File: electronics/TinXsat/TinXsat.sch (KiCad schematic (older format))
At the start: 159 parts, among them J1 USB_B_Mini, J10 CAN, J2 ESP-PROG, J3 POWER_LED, J4 MCO_OUT, J5 BMP280_1, J6 BMP280_2, J7 ESP-card, J8 GPS, J9 SWD, Q1 Si2371, Q2 Si2371, Q3 BSS138, Q4 BSS138, Q5 Si2371, Q6 BSS138, Q7 BSS138, Q8 STD7NK40Z, SW1 SW_Push, U1 CP2102N-A01-GQFN28, U10 TPS61175PWP, U11 STM32F103RGTx, U12 LM35-LP, U13 LM35-LP, U14 LM35-LP, U15 TPS63001, U2 A25L032, U3 MPU-6050, U4 TP4056, U5 Ai-Thinker-Ra-01, U6 ESP32-cam, U7 INA219AxDCN, U8 MCP130, U9 INA219AxDCN, Y1 8Mhz, Y2 32768Hz

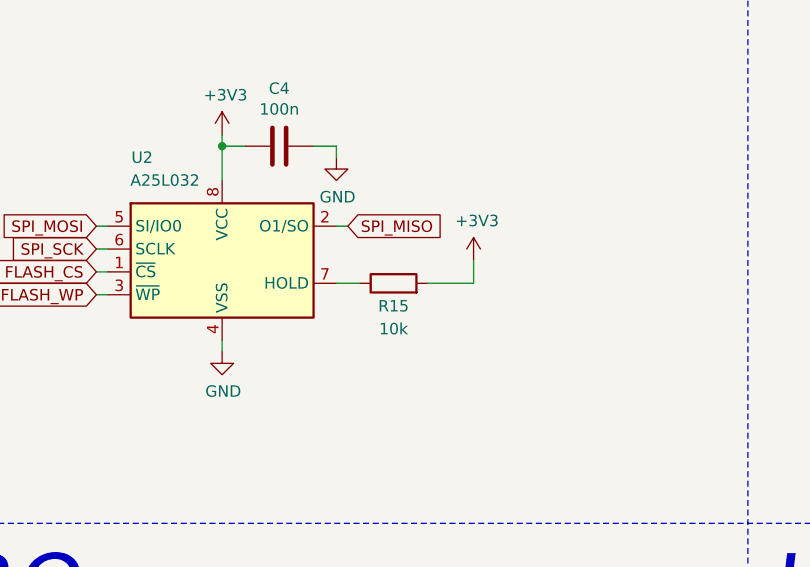
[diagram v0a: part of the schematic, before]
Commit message: pcb gerber commit
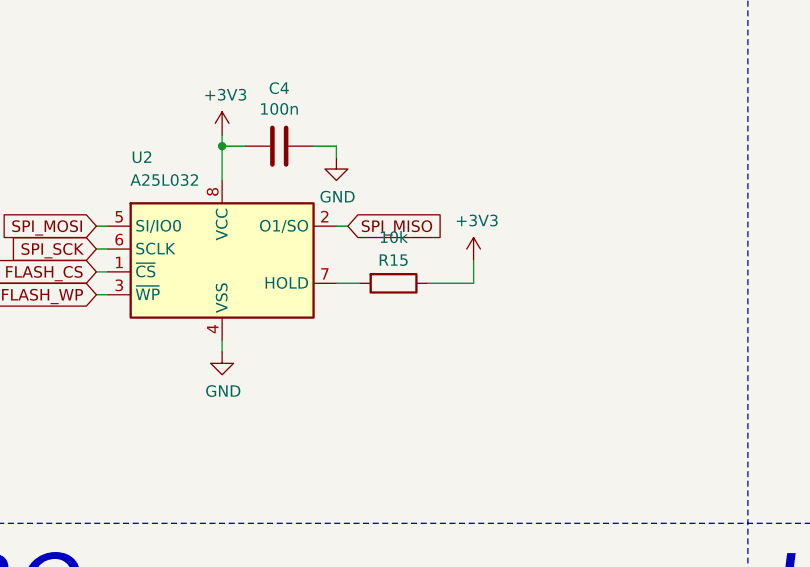
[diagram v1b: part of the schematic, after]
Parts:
- U2: footprint Package_SO:SOP-8_3.9x4.9mm_P1.27mm -> TinXsat:WSON-8-1EP_6x5mm_P1.27mm_EP3.4x4mm
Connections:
- net +3V3: now also R15.1; no longer R15.2
- net at U2.7 (HOLD): now also R15.2; no longer R15.1
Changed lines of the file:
@@
 FLASH_WP
-$Comp
-L sch-lib:A25L032 U2
-U 1 1 60070B82
-P 2250 6750
-F 0 "U2" H 1900 7250 50  0000 C CNN
-F 1 "A25L032" H 2000 7150 50  0000 C CNN
-F 2 "Package_SO:SOP-8_3.9x4.9mm_P1.27mm" H 2250 6150 50  0001 C CNN
-F 3 "http://www.elm-tech.com/en/products/spi-flash-memory/gd25d10/gd25d10.pdf" H 2250 6750 50  0001 C CNN
-	1    2250 6750
-	1    0    0    -1
-$EndComp
 $Comp
 L power:GND #PWR0162
@@
 	1700 6750 1750 6750
 $Comp
-L Device:R R15
-U 1 1 60255FDC
-P 3000 6800
-F 0 "R15" V 2900 6800 50  0000 C CNN
-F 1 "10k" V 2800 6800 50  0000 C CNN
-F 2 "Resistor_SMD:R_0805_2012Metric_Pad1.20x1.40mm_HandSolder" V 2930 6800 50  0001 C CNN
-F 3 "~" H 3000 6800 50  0001 C CNN
-	1    3000 6800
-	0    -1   -1   0
-$EndComp
-$Comp
 L power:+3V3 #PWR0159
 U 1 1 60256D6F
@@
 Wire Wire Line
 	3350 6700 3350 6800
-Wire Wire Line
-	3350 6800 3150 6800
-Wire Wire Line
-	2850 6800 2750 6800
 Wire Wire Line
 	1700 6850 1750 6850
@@
 Wire Wire Line
 	21300 13600 21300 13800
+$Comp
+L Device:R R15
+U 1 1 60130731
+P 3000 6800
+F 0 "R15" V 2900 6800 50  0000 C CNN
+F 1 "10k" V 2800 6800 50  0000 C CNN
+F 2 "Resistor_SMD:R_0805_2012Metric_Pad1.20x1.40mm_HandSolder" V 2930 6800 50  0001 C CNN
+F 3 "~" H 3000 6800 50  0001 C CNN
+	1    3000 6800
+	0    1    1    0
+$EndComp
+Wire Wire Line
+	3150 6800 3350 6800
+Wire Wire Line
+	2750 6800 2850 6800
+$Comp
+L sch-lib:A25L032 U2
+U 1 1 60070B82
+P 2250 6750
+F 0 "U2" H 1900 7250 50  0000 C CNN
+F 1 "A25L032" H 2000 7150 50  0000 C CNN
+F 2 "TinXsat:WSON-8-1EP_6x5mm_P1.27mm_EP3.4x4mm" H 2250 6150 50  0001 C CNN
+F 3 "http://www.elm-tech.com/en/products/spi-flash-memory/gd25d10/gd25d10.pdf" H 2250 6750 50  0001 C CNN
+	1    2250 6750
+	1    0    0    -1
+$EndComp
 $EndSCHEMATC

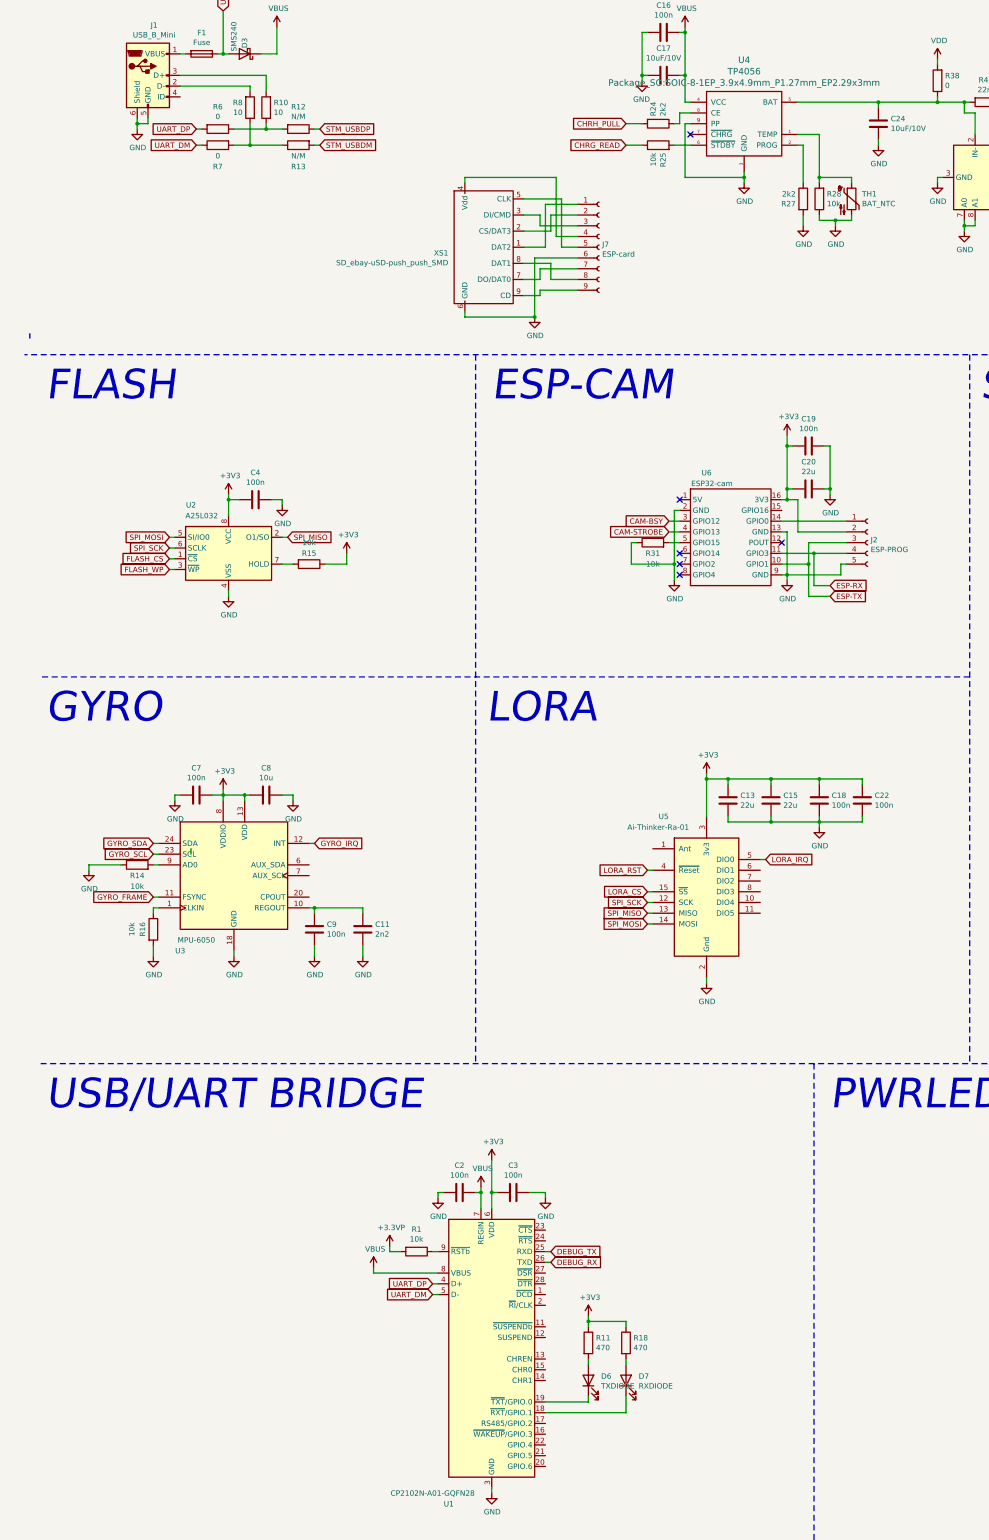
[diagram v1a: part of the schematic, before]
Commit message: pcb final commit after chinese changes
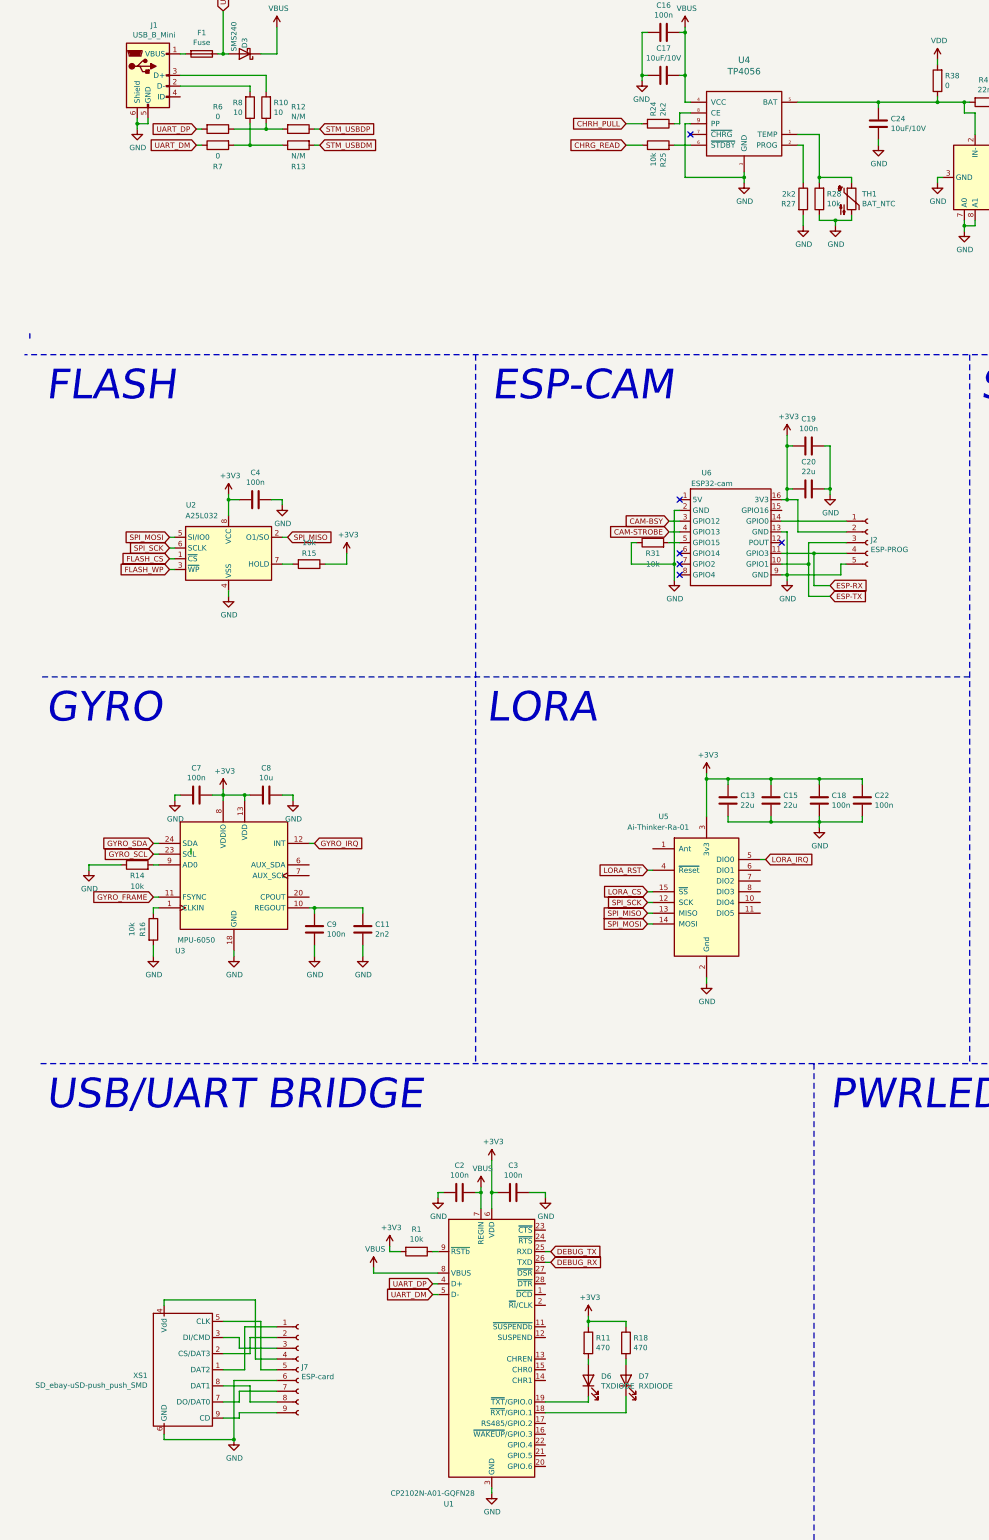
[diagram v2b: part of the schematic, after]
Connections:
- net +3.3VP is gone; now on net +3V3: R1.2
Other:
- moved on the sheet: J7, XS1
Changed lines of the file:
@@
 	4700 12350 4700 12650
 Connection ~ 4700 12650
-$Comp
-L power:+3.3VP #PWR0201
-U 1 1 61CD4E41
-P 3750 13150
-F 0 "#PWR0201" H 3900 13100 50  0001 C CNN
-F 1 "+3.3VP" H 3765 13323 50  0000 C CNN
-F 2 "" H 3750 13150 50  0001 C CNN
-F 3 "" H 3750 13150 50  0001 C CNN
-	1    3750 13150
-	1    0    0    -1
-$EndComp
 Wire Wire Line
 	4150 13200 4200 13200
@@
 F 0 "U4" H 7050 3393 60  0000 C CNN
 F 1 "TP4056" H 7050 3287 60  0000 C CNN
-F 2 "Package_SO:SOIC-8-1EP_3.9x4.9mm_P1.27mm_EP2.29x3mm" H 7050 3181 60  0000 C CNN
+F 2 "Package_SO:SOIC-8-1EP_3.9x4.9mm_P1.27mm_EP2.29x3mm" H 7050 3181 60  0001 C CNN
 F 3 "" H 7050 2750 60  0000 C CNN
 	1    7050 2750
@@
 	20900 11900 21550 11900
 $Comp
-L uSD_push-push_ebay:SD_ebay-uSD-push_push_SMD XS1
-U 1 1 61BF60BB
-P 4600 3950
-F 0 "XS1" H 4296 3996 50  0000 R CNN
-F 1 "SD_ebay-uSD-push_push_SMD" H 4296 3905 50  0000 R CNN
-F 2 "footprints:Conn_uSDcard" H 4600 3950 10  0001 C CNN
-F 3 "_" H 4600 3950 10  0001 C CNN
-F 4 "_" H 4600 3950 10  0001 C CNN "Manf#"
-F 5 "ebay" H 4600 3950 10  0001 C CNN "Manf"
-	1    4600 3950
-	1    0    0    -1
-$EndComp
-$Comp
 L Analog_ADC:INA219AxDCN U7
 U 1 1 6237EB1E
@@
 L Connector:Conn_01x09_Female J7
 U 1 1 5FEDD748
-P 5700 3850
-F 0 "J7" H 5728 3876 50  0000 L CNN
-F 1 "ESP-card" H 5728 3785 50  0000 L CNN
-F 2 "TinXsat:PinHeader_1x08_P2mm_SMD" H 5700 3850 50  0001 C CNN
-F 3 "~" H 5700 3850 50  0001 C CNN
-	1    5700 3850
-	1    0    0    -1
-$EndComp
-Wire Wire Line
-	5200 3450 5200 3850
-Wire Wire Line
-	5200 3850 5000 3850
-Wire Wire Line
-	5200 3450 5500 3450
-Wire Wire Line
-	5500 3550 5250 3550
-Wire Wire Line
-	5250 3550 5250 3700
-Wire Wire Line
-	5250 3700 5000 3700
-Wire Wire Line
-	5000 3550 5150 3550
-Wire Wire Line
-	5150 3550 5150 3650
-Wire Wire Line
-	5150 3650 5500 3650
-Wire Wire Line
-	4450 3250 4450 3200
-Wire Wire Line
-	4450 3200 5300 3200
-Wire Wire Line
-	5300 3200 5300 3750
-Wire Wire Line
-	5300 3750 5500 3750
-Wire Wire Line
-	5500 3850 5350 3850
-Wire Wire Line
-	5350 3850 5350 3400
-Wire Wire Line
-	5350 3400 5000 3400
-Wire Wire Line
-	4450 4450 4450 4500
-Wire Wire Line
-	4450 4500 5100 4500
-Wire Wire Line
-	5100 4500 5100 3950
-Wire Wire Line
-	5100 3950 5500 3950
-Wire Wire Line
-	5500 4050 5150 4050
-Wire Wire Line
-	5150 4050 5150 4150
-Wire Wire Line
-	5150 4150 5000 4150
-Wire Wire Line
-	5000 4000 5250 4000
-Wire Wire Line
-	5250 4000 5250 4150
-Wire Wire Line
-	5250 4150 5500 4150
-Wire Wire Line
-	5500 4250 5150 4250
-Wire Wire Line
-	5150 4250 5150 4300
-Wire Wire Line
-	5150 4300 5000 4300
+P 2900 14300
+F 0 "J7" H 2928 14326 50  0000 L CNN
+F 1 "ESP-card" H 2928 14235 50  0000 L CNN
+F 2 "TinXsat:PinHeader_1x08_P2mm_SMD" H 2900 14300 50  0001 C CNN
+F 3 "~" H 2900 14300 50  0001 C CNN
+	1    2900 14300
+	1    0    0    -1
+$EndComp
+Wire Wire Line
+	2400 13900 2400 14300
+Wire Wire Line
+	2400 14300 2200 14300
+Wire Wire Line
+	2400 13900 2700 13900
+Wire Wire Line
+	2700 14000 2450 14000
+Wire Wire Line
+	2450 14000 2450 14150
+Wire Wire Line
+	2450 14150 2200 14150
+Wire Wire Line
+	2200 14000 2350 14000
+Wire Wire Line
+	2350 14000 2350 14100
+Wire Wire Line
+	2350 14100 2700 14100
+Wire Wire Line
+	1650 13700 1650 13650
+Wire Wire Line
+	1650 13650 2500 13650
+Wire Wire Line
+	2500 13650 2500 14200
+Wire Wire Line
+	2500 14200 2700 14200
+Wire Wire Line
+	2700 14300 2550 14300
+Wire Wire Line
+	2550 14300 2550 13850
+Wire Wire Line
+	2550 13850 2200 13850
+Wire Wire Line
+	1650 14900 1650 14950
+Wire Wire Line
+	1650 14950 2300 14950
+Wire Wire Line
+	2300 14950 2300 14400
+Wire Wire Line
+	2300 14400 2700 14400
+Wire Wire Line
+	2700 14500 2350 14500
+Wire Wire Line
+	2350 14500 2350 14600
+Wire Wire Line
+	2350 14600 2200 14600
+Wire Wire Line
+	2200 14450 2450 14450
+Wire Wire Line
+	2450 14450 2450 14600
+Wire Wire Line
+	2450 14600 2700 14600
+Wire Wire Line
+	2700 14700 2350 14700
+Wire Wire Line
+	2350 14700 2350 14750
+Wire Wire Line
+	2350 14750 2200 14750
 Text GLabel 1700 6850 0    50   Input ~ 0
 FLASH_WP
@@
 L power:GND #PWR0219
 U 1 1 5FF2DAEA
-P 5100 4500
-F 0 "#PWR0219" H 5100 4250 50  0001 C CNN
-F 1 "GND" H 5105 4327 50  0000 C CNN
-F 2 "" H 5100 4500 50  0001 C CNN
-F 3 "" H 5100 4500 50  0001 C CNN
-	1    5100 4500
-	1    0    0    -1
-$EndComp
-Connection ~ 5100 4500
+P 2300 14950
+F 0 "#PWR0219" H 2300 14700 50  0001 C CNN
+F 1 "GND" H 2305 14777 50  0000 C CNN
+F 2 "" H 2300 14950 50  0001 C CNN
+F 3 "" H 2300 14950 50  0001 C CNN
+	1    2300 14950
+	1    0    0    -1
+$EndComp
+Connection ~ 2300 14950
 $Comp
 L power:VDD #PWR0128
@@
 	1    0    0    -1
 $EndComp
+$Comp
+L uSD_push-push_ebay:SD_ebay-uSD-push_push_SMD XS1
+U 1 1 61BF60BB
+P 1800 14400
+F 0 "XS1" H 1496 14446 50  0000 R CNN
+F 1 "SD_ebay-uSD-push_push_SMD" H 1496 14355 50  0000 R CNN
+F 2 "footprints:Conn_uSDcard" H 1800 14400 10  0001 C CNN
+F 3 "_" H 1800 14400 10  0001 C CNN
+F 4 "_" H 1800 14400 10  0001 C CNN "Manf#"
+F 5 "ebay" H 1800 14400 10  0001 C CNN "Manf"
+	1    1800 14400
+	1    0    0    -1
+$EndComp
+$Comp
+L power:+3V3 #PWR?
+U 1 1 5FF40037
+P 3750 13150
+F 0 "#PWR?" H 3750 13000 50  0001 C CNN
+F 1 "+3V3" H 3765 13323 50  0000 C CNN
+F 2 "" H 3750 13150 50  0001 C CNN
+F 3 "" H 3750 13150 50  0001 C CNN
+	1    3750 13150
+	1    0    0    -1
+$EndComp
